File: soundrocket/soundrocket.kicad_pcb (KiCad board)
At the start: 4 copper layers, 92.7 x 45.7 mm, 12 parts, among them J1 XLR3 MALE (OUT), SW1 SW_Push, SW2 RotaryEncoder_Switch, T1 PE-65612NL, U1 Teensy4.0, U2 DIT4192IPW

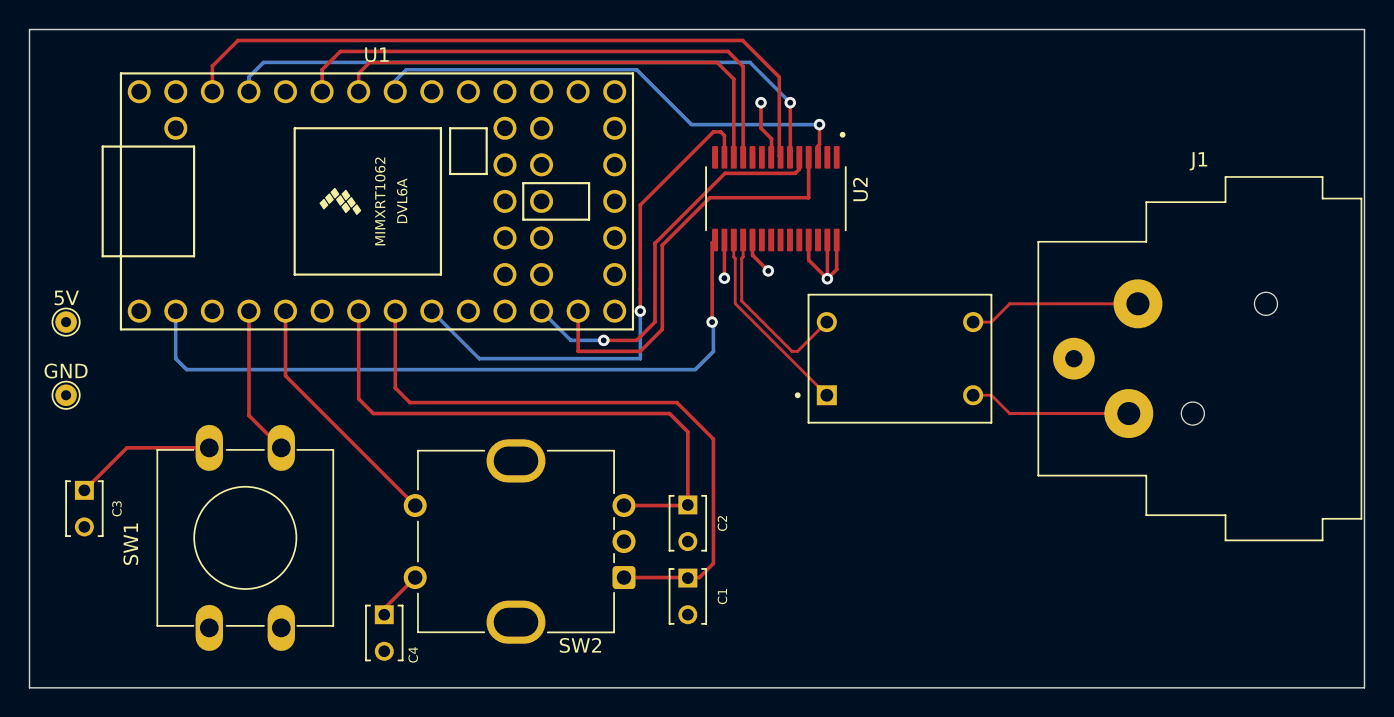
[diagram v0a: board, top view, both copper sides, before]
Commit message: soundbullet format
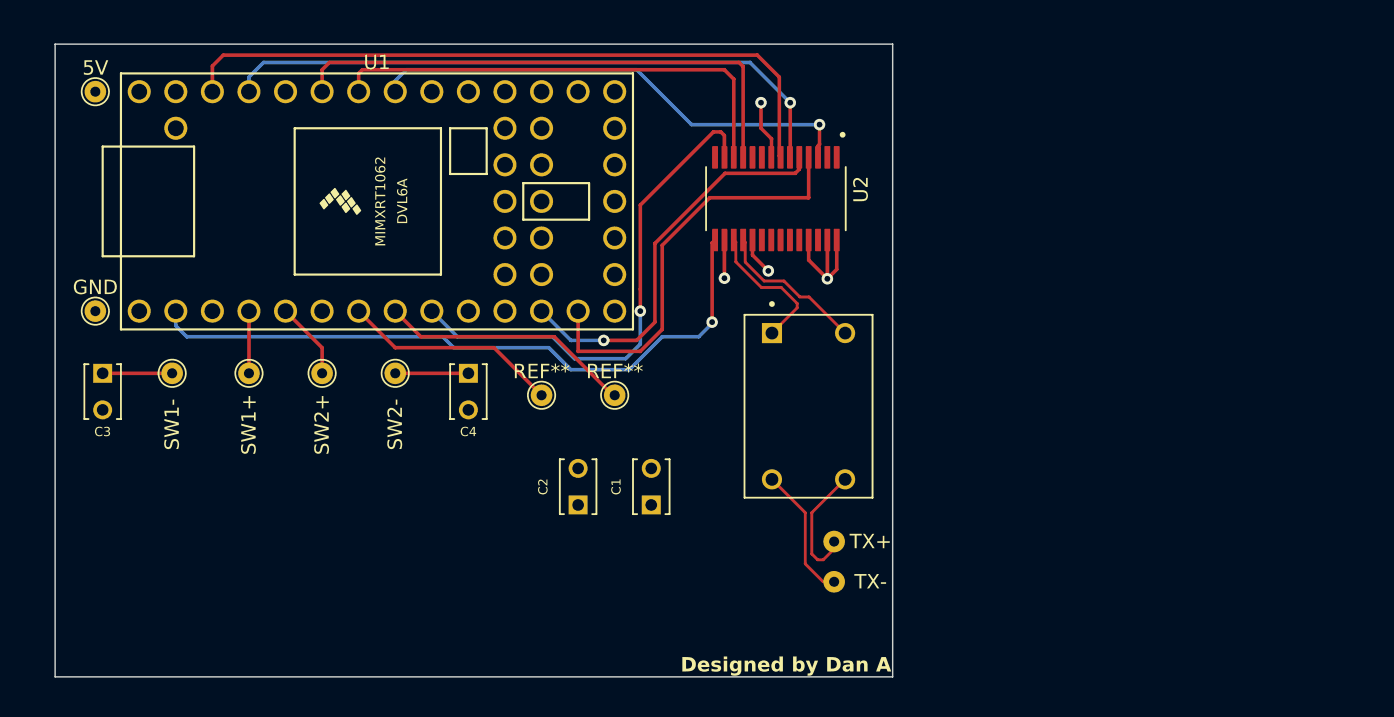
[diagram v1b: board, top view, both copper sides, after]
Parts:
- removed J1: XLR3 MALE (OUT), Connector_Audio:Jack_XLR_Neutrik_NC3FAAH-0_Horizontal
- removed SW1: SW_Push, Button_Switch_THT:SW_PUSH-12mm
- removed SW2: RotaryEncoder_Switch, Rotary_Encoder:RotaryEncoder_Bourns_Vertical_PEC12R-3x17F-Sxxxx
- added ?: , , F.Cu at (175.3, 66.3)
- added ?: , , F.Cu at (175.3, 63.5)
- added REF**: TestPoint_THTPad_D1.5mm_Drill0.7mm, TestPoint:TestPoint_THTPad_D1.5mm_Drill0.7mm, F.Cu at (160.0, 53.3)
- added REF**: TestPoint_THTPad_D1.5mm_Drill0.7mm, TestPoint:TestPoint_THTPad_D1.5mm_Drill0.7mm, F.Cu at (154.9, 53.3)
- added SW1+: TestPoint_THTPad_D1.5mm_Drill0.7mm, TestPoint:TestPoint_THTPad_D1.5mm_Drill0.7mm, F.Cu at (134.6, 51.8)
- added SW1-: TestPoint_THTPad_D1.5mm_Drill0.7mm, TestPoint:TestPoint_THTPad_D1.5mm_Drill0.7mm, F.Cu at (129.3, 51.8)
- added SW2+: TestPoint_THTPad_D1.5mm_Drill0.7mm, TestPoint:TestPoint_THTPad_D1.5mm_Drill0.7mm, F.Cu at (139.7, 51.8)
- added SW2-: TestPoint_THTPad_D1.5mm_Drill0.7mm, TestPoint:TestPoint_THTPad_D1.5mm_Drill0.7mm, F.Cu at (144.8, 51.8)
- moved C4 17.8 mm to (149.9, 53.1)
- moved 5V 16.1 mm to (124.0, 32.3)
- moved C3 8.23 mm to (124.5, 53.1)
- moved C2 8.03 mm to (157.5, 59.7), turned to 90 degrees
- moved C1 8.03 mm to (162.6, 59.7), turned to 90 degrees
- moved T1 7.16 mm to (173.5, 54.1), turned to -90 degrees
- moved GND 6.19 mm to (124.0, 47.5)
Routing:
- net Net-(U1-6_OUT1D): track 44.2 -> 17.7 mm
- net Net-(U1-5_IN2): track 39.4 -> 15.1 mm
- net Net-(U1-3_LRCLK2): track 17.2 -> 5.37 mm
- net Net-(U1-2_OUT2): track 10.4 -> 4.32 mm
- net Net-(C3-Pad1): track 9.90 -> 4.83 mm
- net /DIT4192-TX-: track 13.5 -> 9.82 mm
- net /XLR-TX+: track 12.0 -> 8.68 mm
- net Net-(U1-0_RX1_CRX2_CS1): track 49.3 -> 46.7 mm
- net /XLR-TX-: track 11.3 -> 9.35 mm
- net /DIT4192-TX+: track 12.5 -> 10.6 mm
- net Net-(C4-Pad1): track 3.47 -> 5.08 mm
- net Net-(U2-V_IO): track 48.5 -> 47.7 mm
- net Net-(U1-21_A7_RX5_BCLK1): track 38.0 -> 37.4 mm
- net Net-(U1-7_RX2_OUT1A): track 36.1 -> 35.5 mm
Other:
- board size 92.7 x 45.7 mm -> 58.2 x 43.9 mm
- board text added: "Designed by Dan A"
- board text added: "TX+"
- board text added: "TX-"
- board text removed: "Design by Daniel Anderson"
